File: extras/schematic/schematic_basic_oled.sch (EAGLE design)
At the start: 18 parts, among them U1 SI4735-D60-GU

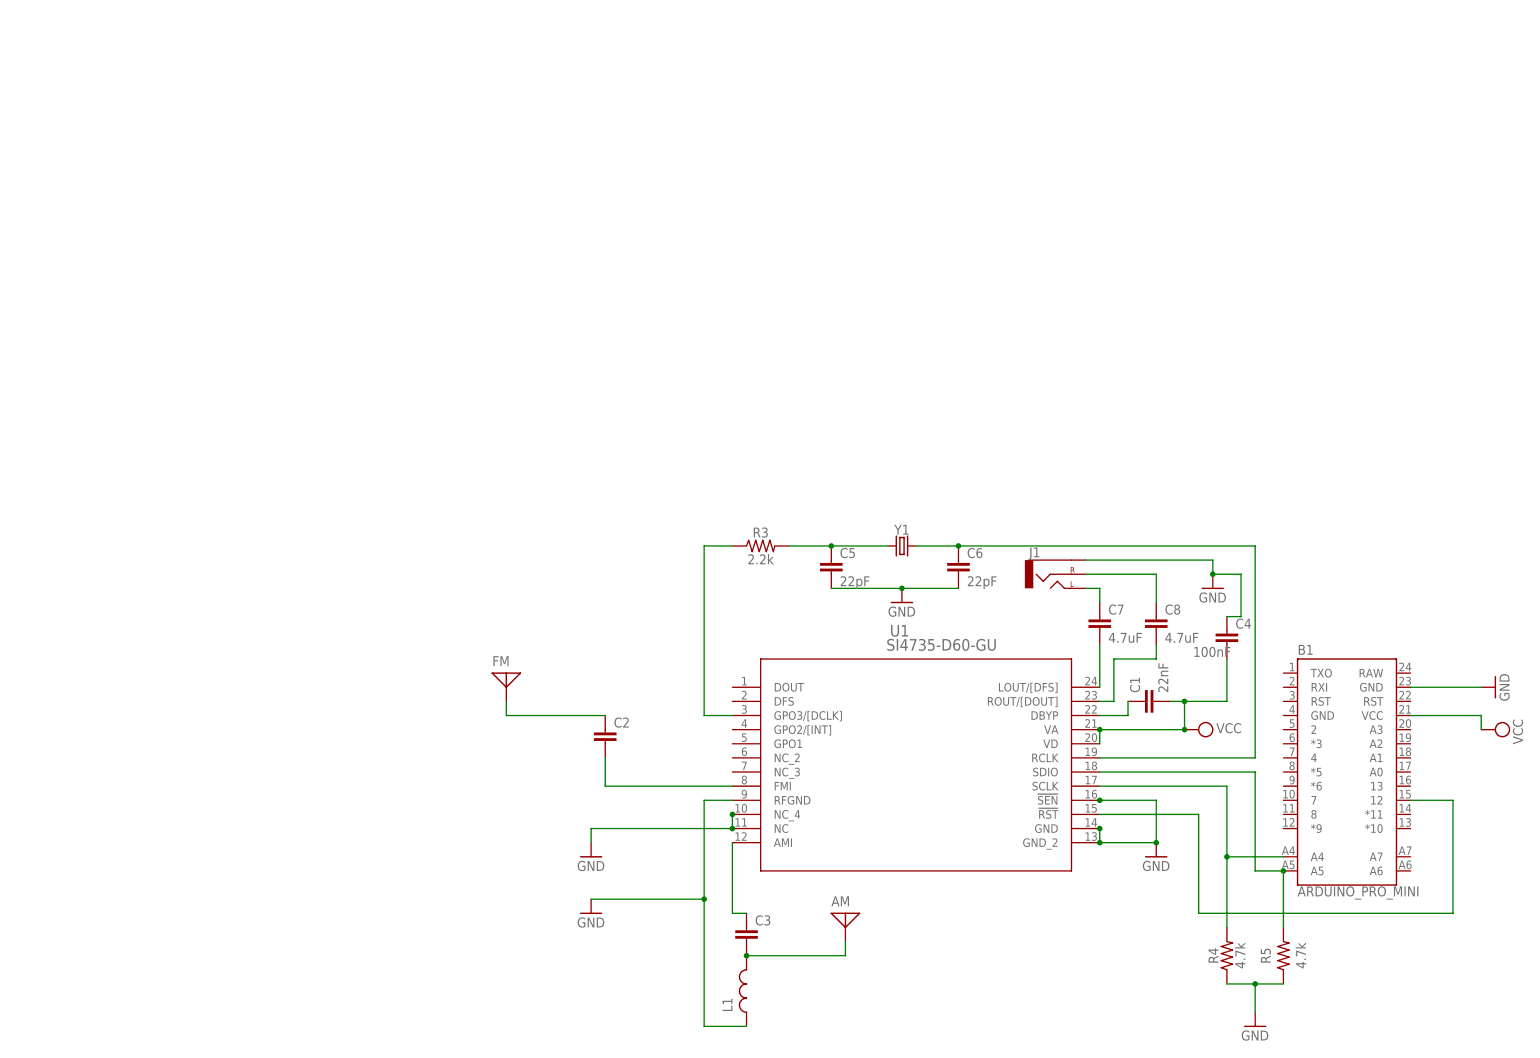
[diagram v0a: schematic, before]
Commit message: SI47XX Arduino Library
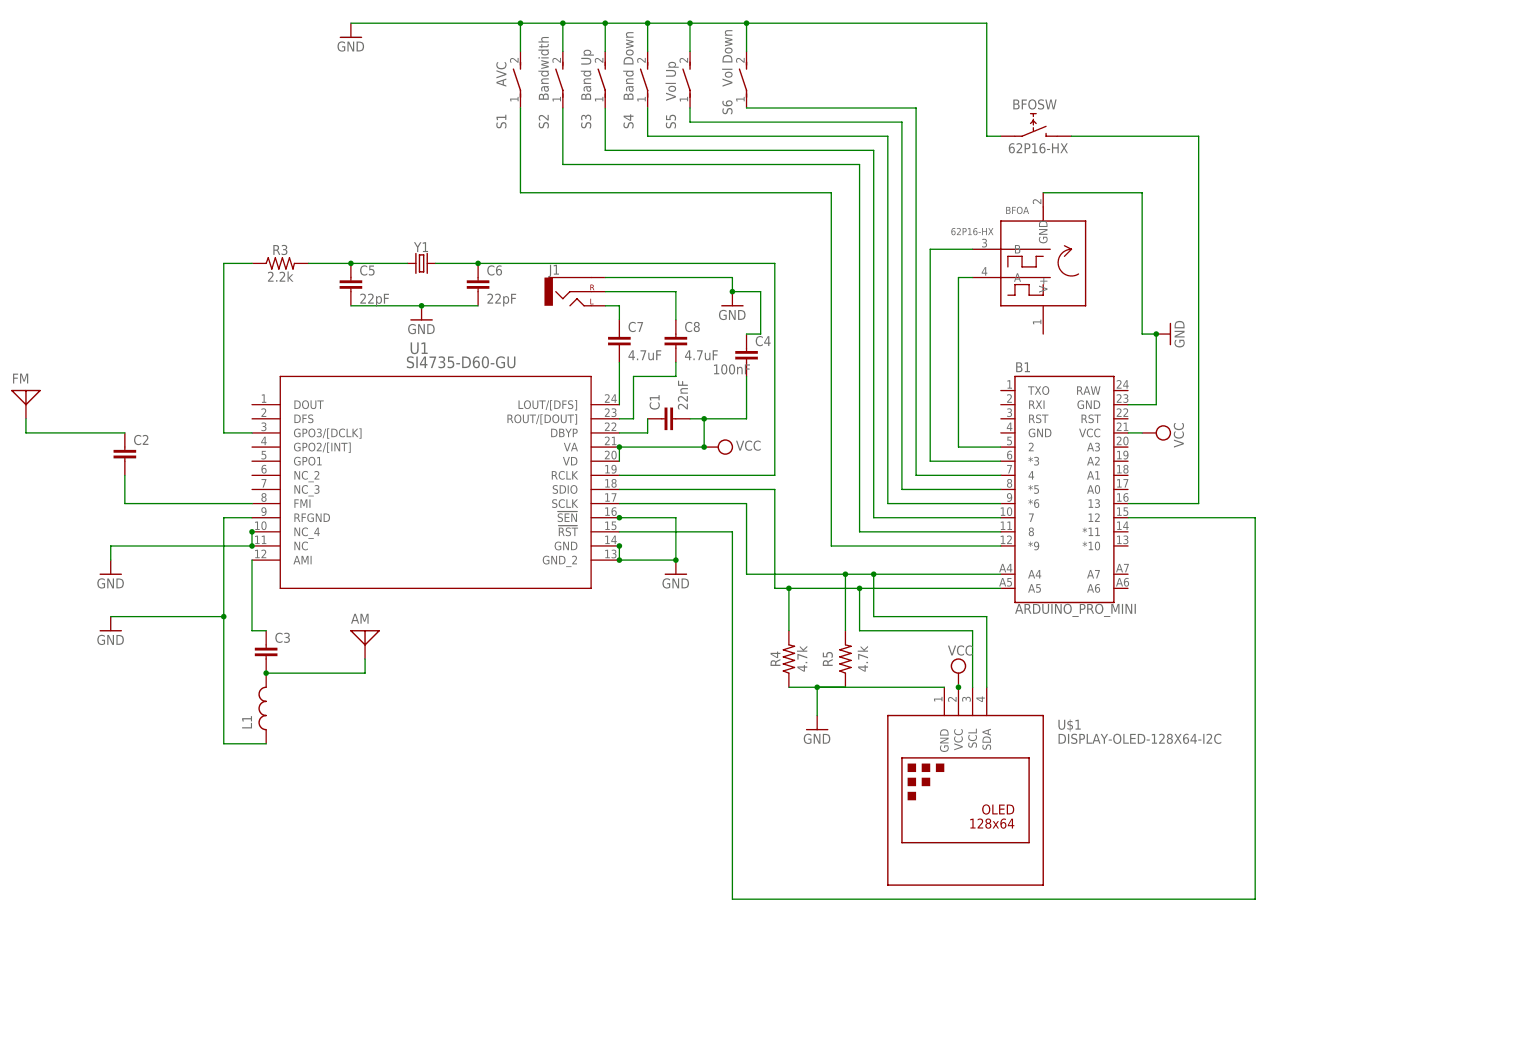
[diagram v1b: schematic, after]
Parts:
- added BFO: 62P16-HX, rotary-encoder:62P16-HX
- added S1: AVC, switch-dil:DS01E
- added S2: Bandwidth, switch-dil:DS01E
- added S3: Band Up, switch-dil:DS01E
- added S4: Band Down, switch-dil:DS01E
- added S5: Vol Up, switch-dil:DS01E
- added S6: Vol Down, switch-dil:DS01E
- added U$1: DISPLAY-OLED-128X64-I2C, diy-modules:DISPLAY-OLED-128X64-I2C
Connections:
- new net N$15: B1.2, BFOA.A
- new net N$16: B1.*3, BFOA.B
- new net N$17: B1.4, S6.1
- new net N$18: B1.*5, S5.1
- new net N$19: B1.*6, S4.1
- new net N$20: B1.7, S3.1
- new net N$21: B1.8, S2.1
- new net N$22: B1.*9, S1.1
- new net N$24: B1.13, BFOSW.E
- net GND: now also BFOA.GND, BFOSW.D, S1.2, S2.2, S3.2, S4.2, S5.2, S6.2, U$1.GND
- net N$2: now also R5.2, U$1.SDA; no longer R4.2
- net SDA: now also R4.2, U$1.SCL; no longer R5.2
- net VCC: now also U$1.VCC
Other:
- moved on the sheet: AM, B1, C1, C2, C3, C4, C5, C6, C7, C8, FM, J1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
